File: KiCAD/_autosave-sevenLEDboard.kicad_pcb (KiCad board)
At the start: 2 copper layers, 23.1 x 20 mm, 14 parts, among them J1 Conn_01x03_Male, U1 SC4541

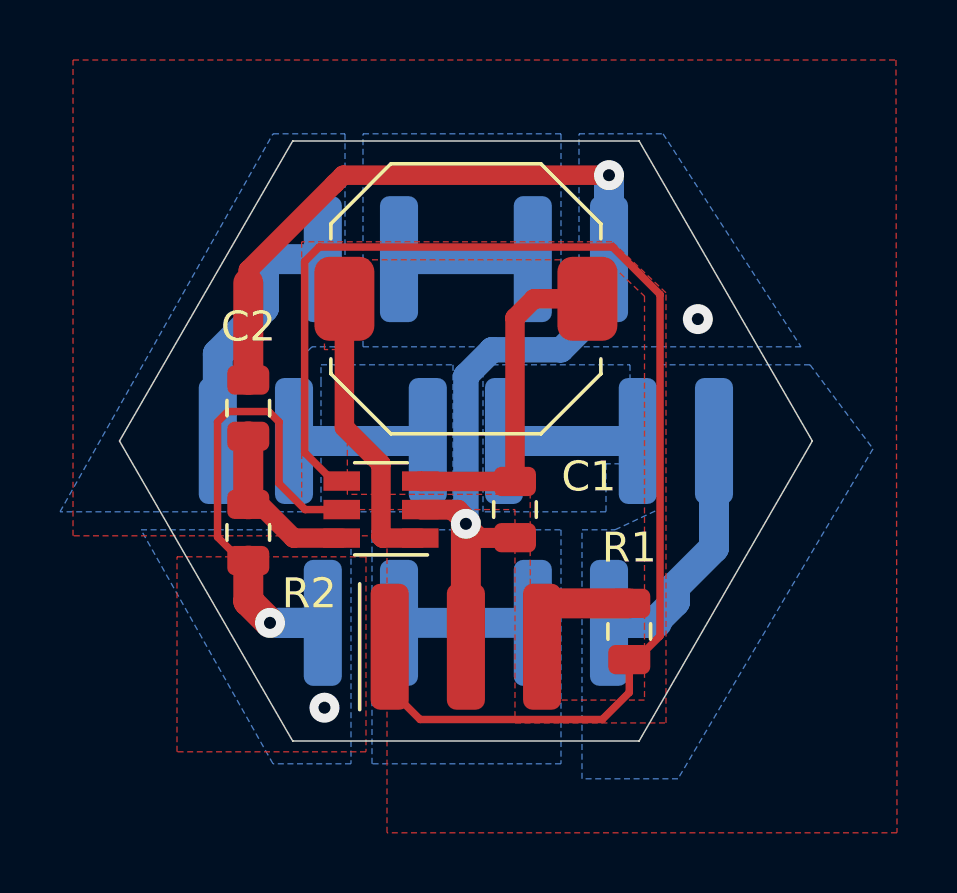
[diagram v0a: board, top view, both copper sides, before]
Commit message: Final changes with fabrication outputs.
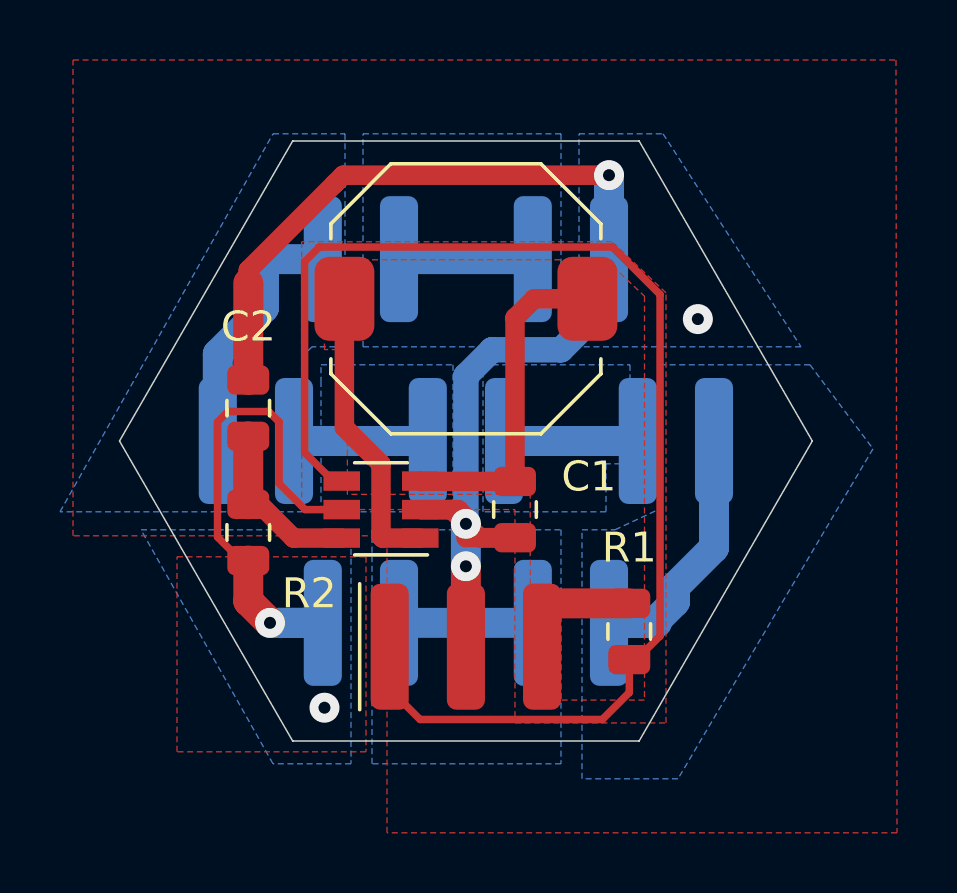
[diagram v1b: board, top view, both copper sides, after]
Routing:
- net GND: vias 3 -> 4
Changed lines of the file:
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@@
     (thickness 1.6)
     (drawings 6)
-    (tracks 86)
+    (tracks 88)
     (zones 0)
     (modules 14)
@@
     (visible_elements 7FFFFFFF)
     (pcbplotparams
-      (layerselection 0x010fc_ffffffff)
+      (layerselection 0x010d0_ffffffff)
       (usegerberextensions false)
       (usegerberattributes true)
@@
   (segment (start 145.8935 81.9635) (end 145.43 81.5) (width 0.65) (layer F.Cu) (net 1))
   (segment (start 147.066 81.9635) (end 145.8935 81.9635) (width 0.65) (layer F.Cu) (net 1))
-  (segment (start 145.43 85.598) (end 145.43 81.5) (width 1) (layer F.Cu) (net 1))
+  (segment (start 145.43 85.598) (end 145.43 82.916) (width 1) (layer F.Cu) (net 1))
   (via (at 153.162 74.676) (size 1) (drill 0.4) (layers F.Cu B.Cu) (net 1))
+  (via (at 145.43 82.916) (size 1) (drill 0.4) (layers F.Cu B.Cu) (net 1))
+  (segment (start 145.43 81.5) (end 145.43 82.916) (width 1) (layer B.Cu) (net 1))
   (segment (start 146.5375 80.076) (end 146.55 80.0885) (width 0.25) (layer F.Cu) (net 2))
   (segment (start 143.55 80.076) (end 146.5375 80.076) (width 0.25) (layer F.Cu) (net 2))
